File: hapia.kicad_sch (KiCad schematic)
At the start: 89 parts, among them CN1 100nf, CN2 100nf, J1 Conn_ARM_JTAG_SWD_10, J2 USB_C_Receptacle_USB2.0_16P, SW1 SW_Push, SW2 SW_Push, U1 STM32F407VET6, U2 AMS1117-3.3, U3 SRV05-4, Y1 8mhz

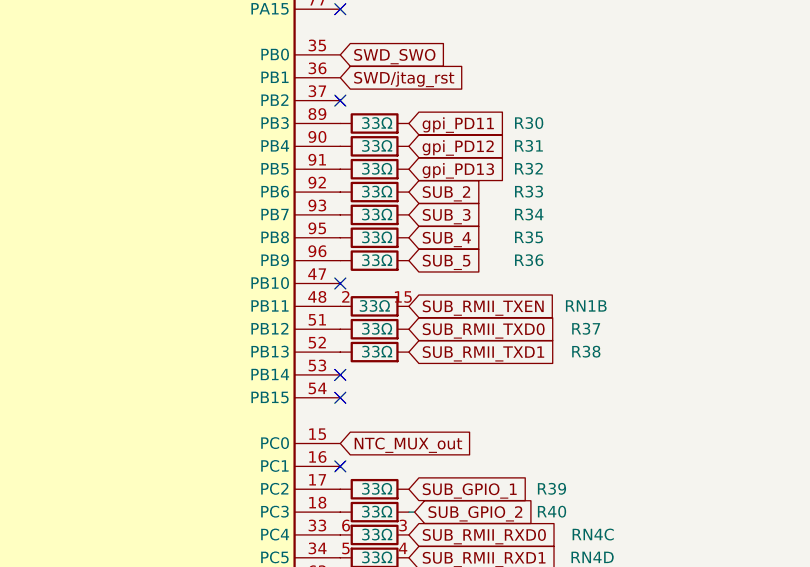
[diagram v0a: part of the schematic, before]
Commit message: 23082026/H
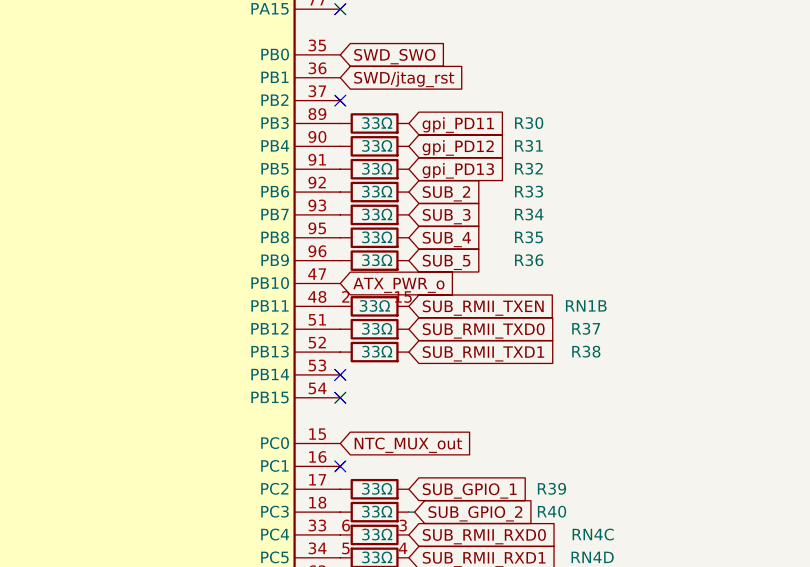
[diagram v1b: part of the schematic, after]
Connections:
- net ATX_PWR_o: now reaches U1.47 (PB10)
- no-connect marks 23 -> 22
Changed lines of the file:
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@@
-	)
-	(no_connect
-		(at 128.27 163.83)
 	)
 	(no_connect
@@
 			(hide yes)
 			(show_name no)
+			(do_not_autoplace no)
+			(effects
+				(font
+					(size 1.27 1.27)
+				)
+				(justify left)
+			)
+		)
+	)
+	(global_label "ATX_PWR_o"
+		(shape input)
+		(at 128.27 163.83 0)
+		(fields_autoplaced yes)
+		(effects
+			(font
+				(size 1.27 1.27)
+			)
+			(justify left)
+		)
+		(property "Intersheetrefs" "${INTERSHEET_REFS}"
+			(at 141.5965 163.83 0)
+			(hide yes)
+			(show_name no)

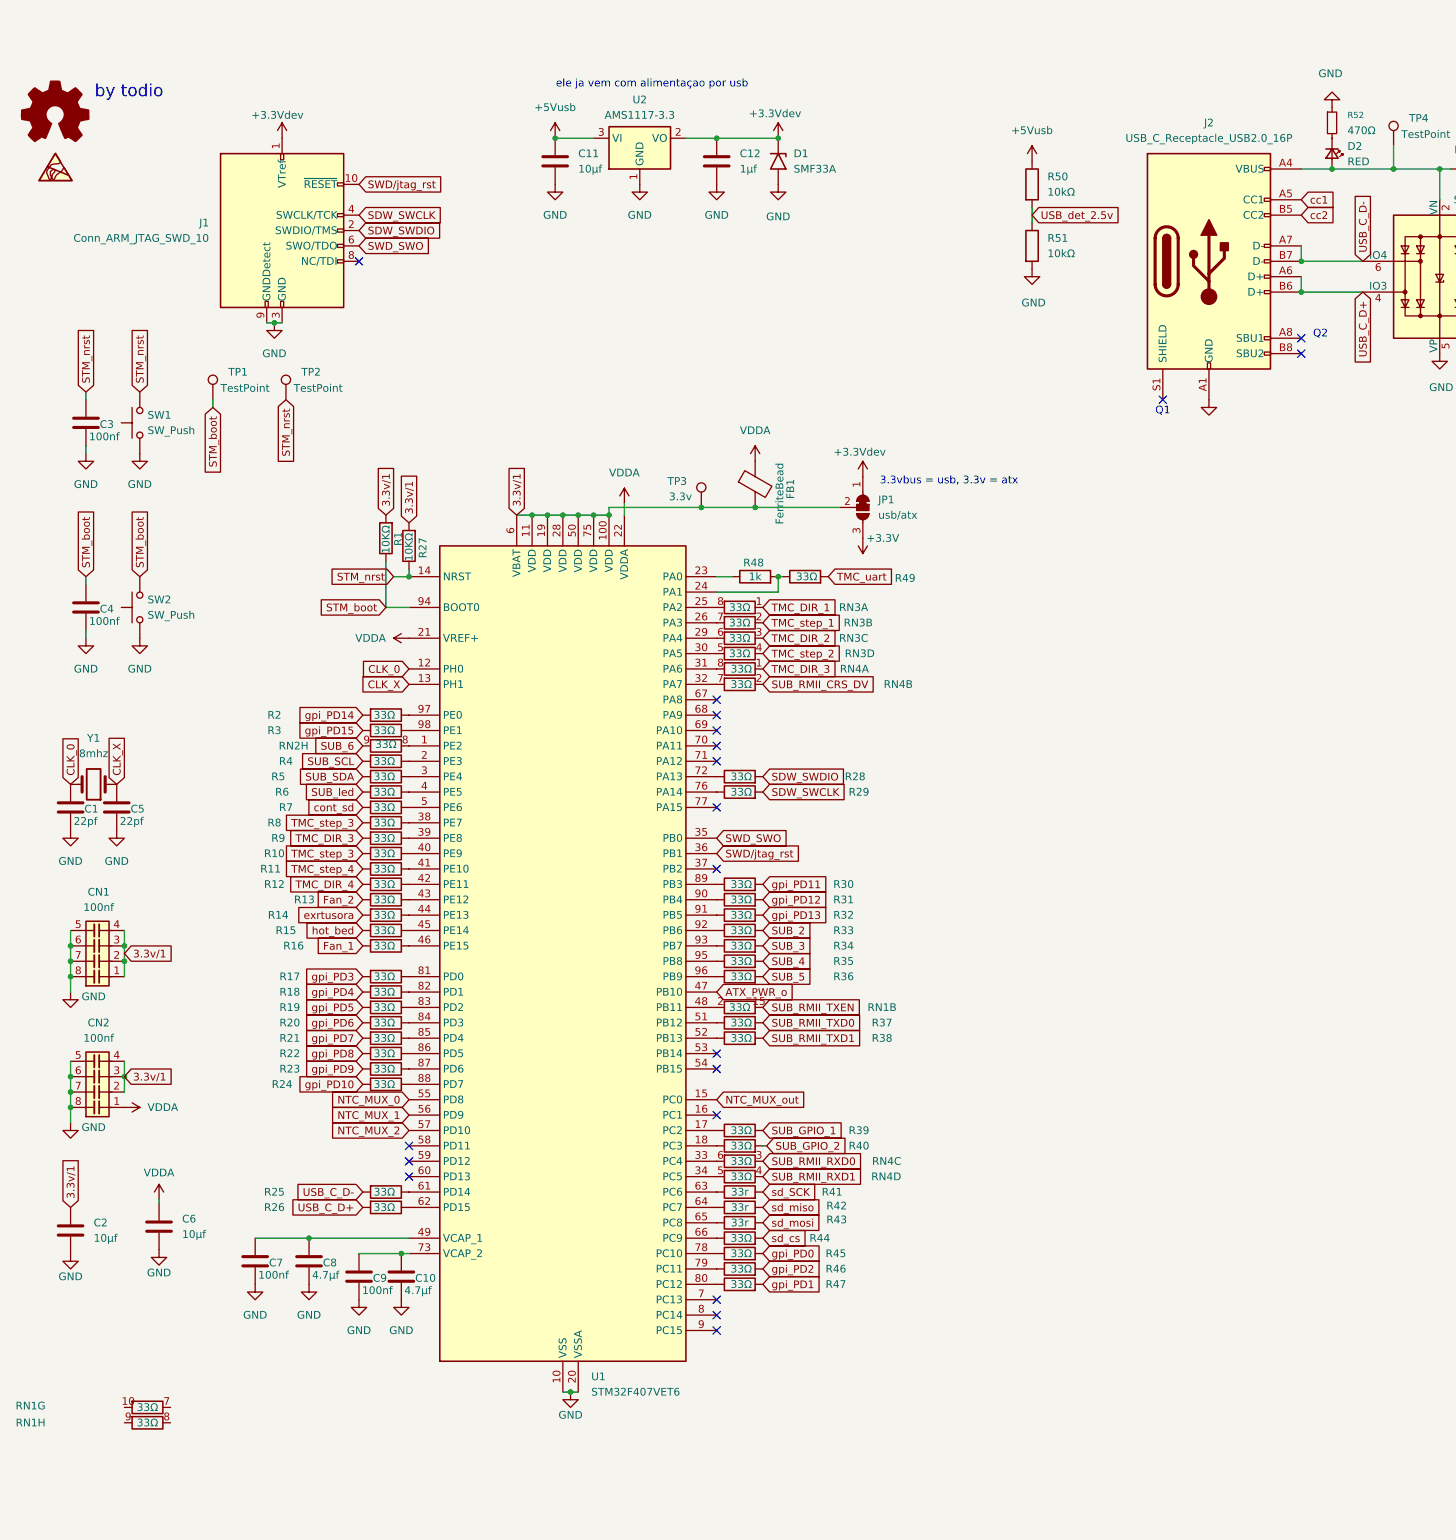
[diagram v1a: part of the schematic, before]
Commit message: 29082026/I
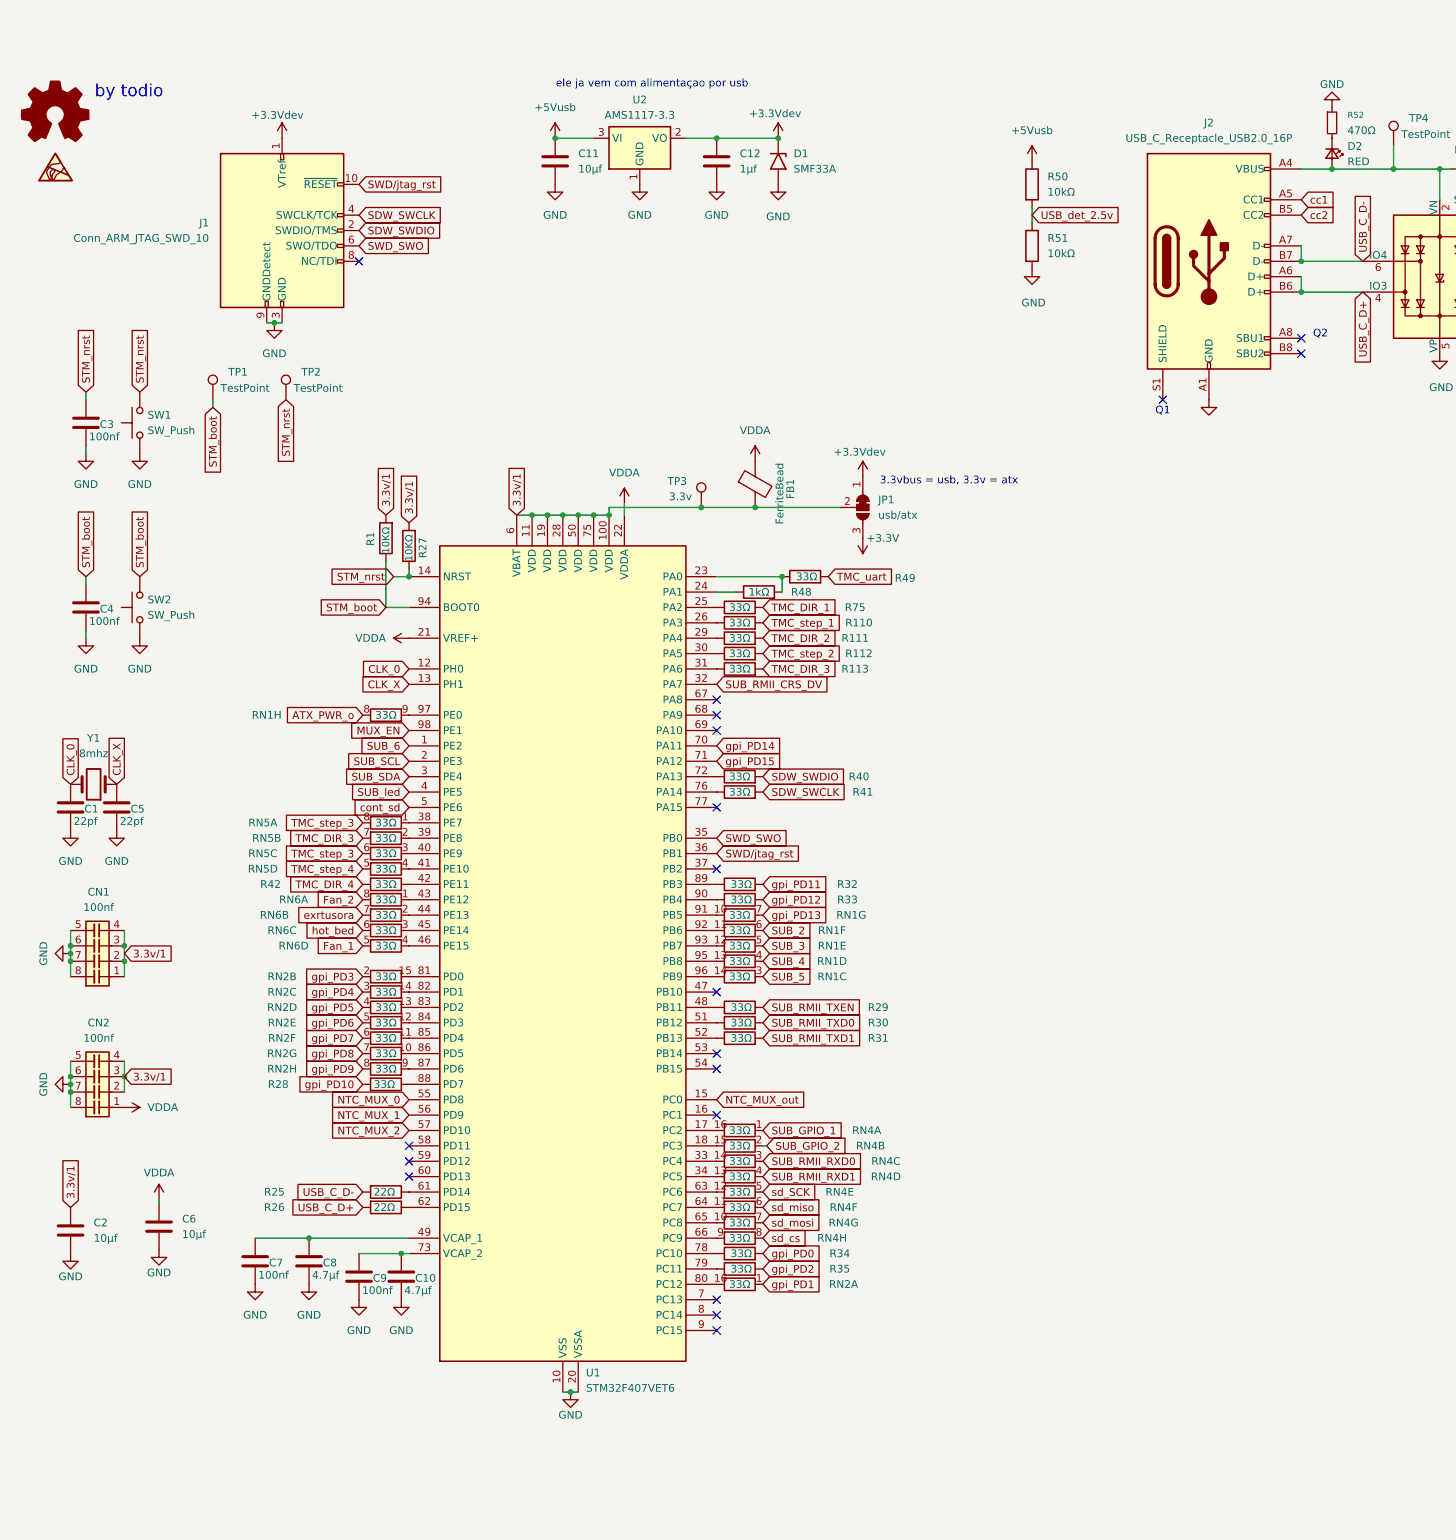
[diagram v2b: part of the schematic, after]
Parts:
- removed R10, R11, R12, R13, R14, R15, R16, R17, R18, R19, R2, R20, R21, R22, R23, R24, R3, R36, R37, R38, R39, R4, R44, R45, R46, R47, R5, R6, R7, R8, R9: 33Ω, symbol Device:R
- removed R43: 33r, symbol Device:R
- removed unit 2 of RN1
- removed RN3, RN4: 33Ω, Resistor_SMD:R_Array_Convex_4x0603, symbol Device:R_Pack04_Split
- added R110, R111, R112, R113, R75: 33Ω, symbol Device:R
- added unit 4 of RN1
- added unit 6 of RN1
- added unit 3 of RN1
- added unit 5 of RN1
- added unit 4 of RN2
- added unit 6 of RN2
- added unit 1 of RN2
- added unit 2 of RN2
- added unit 3 of RN2
- added unit 7 of RN2
- added unit 5 of RN2
- added RN4: 33Ω, symbol Device:R_Pack08_Split
- added RN5, RN6: 33Ω, Resistor_SMD:R_Array_Concave_4x0402, symbol Device:R_Pack04_Split
- C10: footprint (none) -> Capacitor_SMD:C_0603_1608Metric; jlc_pcb: (none) -> C162274; mouser: (none) -> 81-GRM188R61E475KE1D; mpn (none) -> GRM188R61E475KE11D
- C11, C2: footprint (none) -> Capacitor_SMD:C_1206_3216Metric_Pad1.33x1.80mm_HandSolder; jlc_pcb: (none) -> C13585; mouser: (none) -> 187-CL31B106KLK6PNE; mpn (none) -> CL31A106KBHNNNE
- C3, C4, C7, C9: jlc_pcb: C346191 -> C307348; mouser: (none) -> 187-CL10B104KB8WPNC; mpn CL10B104KB8NFNC -> CL10B104KB8WPNC
- C6: footprint (none) -> Capacitor_SMD:C_1206_3216Metric_Pad1.33x1.80mm_HandSolder; Descrição (none) -> esse capacitor e conectado entre o gnd e o vcc(VDDA) do ci 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; jlc_pcb: (none) -> C13585; mouser: (none) -> 187-CL31B106KLK6PNE; mpn (none) -> CL31A106KBHNNNE
- C8: footprint (none) -> Capacitor_SMD:C_0603_1608Metric; Descrição (none) -> capacitor ceramico 4.7uf(µf); jlc_pcb: (none) -> C162274; mouser: (none) -> 81-GRM188R61E475KE1D; mpn (none) -> GRM188R61E475KE11D
- CN1, CN2: jlc_pcb: C346191 -> C307348; mouser: (none) -> 187-CL10B104KB8WPNC; mpn CA0612MRX7R7BB104 -> CL10B104KB8WPNC
- J2: footprint (none) -> Connector_USB:USB_C_Receptacle_HCTL_HC-TYPE-C-16P-01A; jlc_pcb: (none) -> C5150972; mouser: (none) -> 523-12402012E212A; mpn (none) -> 12402012E212A
- R25, R26: value 33Ω -> 22Ω
- R41, R42: value 33r -> 33Ω
- R48: value 1k -> 1kΩ
- RN1, RN2: footprint Resistor_SMD:R_Array_Convex_8x0602 -> (none)
- U1: mouser: (none) -> 511-STM32F407VET6
- U2: mouser: (none) -> 926-LM1117MPX3.3NOPB
- Y1: mouser: (none) -> 815-ABM3-8-D2Y-T
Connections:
- net ATX_PWR_o: now also RN1.8 (R8.1); no longer U1.47 (PB10)
- net Fan_1: now also RN6.5 (R4.2)
- net Fan_2: now also RN6.8 (R1.2)
- net SDW_SWCLK: now also R41.2; no longer R29.2
- net SDW_SWDIO: now also R40.2; no longer R28.2
- net SUB_2: now also RN1.6 (R6.1); no longer R33.2
- net SUB_3: now also RN1.5 (R5.1); no longer R34.2
- net SUB_4: now also RN1.4 (R4.1); no longer R35.2
- net SUB_5: now also RN1.3 (R3.1)
- net SUB_6: now also U1.1 (PE2); no longer RN2.9 (R8.2)
- net SUB_GPIO_1: now also RN4.1 (R1.1)
- net SUB_GPIO_2: now also RN4.2 (R2.1); no longer R40.2
- net SUB_RMII_CRS_DV: now also U1.32 (PA7)
- net SUB_RMII_RXD0: now also RN4.3 (R3.1)
- net SUB_RMII_RXD1: now also RN4.4 (R4.1)
- net SUB_RMII_TXD0: now also R30.2
- net SUB_RMII_TXD1: now also R31.2
- net SUB_RMII_TXEN: now also R29.2
- net SUB_SCL: now also U1.2 (PE3)
- net SUB_SDA: now also U1.3 (PE4)
- net SUB_led: now also U1.4 (PE5)
- net TMC_DIR_1: now also R75.2
- net TMC_DIR_2: now also R111.2
- net TMC_DIR_3: now also R113.2, RN5.7 (R2.2)
- net TMC_DIR_4: now also R42.2
- net TMC_step_1: now also R110.2
- net TMC_step_2: now also R112.2
- net TMC_step_3: now also RN5.6 (R3.2), RN5.8 (R1.2)
- net TMC_step_4: now also RN5.5 (R4.2)
- net cont_sd: now also U1.5 (PE6)
- net exrtusora: now also RN6.7 (R2.2)
- net gpi_PD0: now also R34.2
- net gpi_PD1: now also RN2.1 (R1.1)
- net gpi_PD10: now also R28.2
- net gpi_PD11: now also R32.2; no longer R30.2
- net gpi_PD12: now also R33.2; no longer R31.2
- net gpi_PD13: now also RN1.7 (R7.1); no longer R32.2
- net gpi_PD14: now also U1.70 (PA11)
- net gpi_PD15: now also U1.71 (PA12)
- net gpi_PD2: now also R35.2
- net gpi_PD3: now also RN2.2 (R2.1)
- net gpi_PD4: now also RN2.3 (R3.1)
- net gpi_PD5: now also RN2.4 (R4.1)
- net gpi_PD6: now also RN2.5 (R5.1)
- net gpi_PD7: now also RN2.6 (R6.1)
- net gpi_PD8: now also RN2.7 (R7.1)
- net gpi_PD9: now also RN2.8 (R8.1)
- net hot_bed: now also RN6.6 (R3.2)
- net sd_SCK: now also RN4.5 (R5.1); no longer R41.2
- net sd_cs: now also RN4.8 (R8.1)
- net sd_miso: now also RN4.6 (R6.1); no longer R42.2
- net sd_mosi: now also RN4.7 (R7.1)
- net at U1.52 (PB13): now also R31.1
- net at U1.43 (PE12): now also RN6.1 (R1.1)
- net at U1.65 (PC8): now also RN4.10 (R7.2)
- net at U1.79 (PC11): now also R35.1
- net at U1.38 (PE7): now also RN5.1 (R1.1)
- net at U1.48 (PB11): now also R29.1
- net at U1.85 (PD4): now also RN2.11 (R6.2)
- net at U1.18 (PC3): now also RN4.15 (R2.2); no longer R40.1
- net at U1.26 (PA3): now also R110.1
- net at U1.51 (PB12): now also R30.1
- net at U1.89 (PB3): now also R32.1; no longer R30.1
- net at U1.88 (PD7): now also R28.1
- net at R48.1: now also U1.24 (PA1); no longer U1.23 (PA0)
- net at R48.2, R49.1: now also U1.23 (PA0); no longer U1.24 (PA1)
- net at U1.17 (PC2): now also RN4.16 (R1.2)
- net at U1.25 (PA2): now also R75.1
- net at U1.29 (PA4): now also R111.1
- net at U1.30 (PA5): now also R112.1
- net at U1.31 (PA6): now also R113.1
- net at U1.33 (PC4): now also RN4.14 (R3.2)
- net at U1.34 (PC5): now also RN4.13 (R4.2)
- net at U1.39 (PE8): now also RN5.2 (R2.1)
- net at U1.40 (PE9): now also RN5.3 (R3.1)
- net at U1.41 (PE10): now also RN5.4 (R4.1)
- net at U1.42 (PE11): now also R42.1
- net at U1.44 (PE13): now also RN6.2 (R2.1)
- net at U1.45 (PE14): now also RN6.3 (R3.1)
- net at U1.46 (PE15): now also RN6.4 (R4.1)
- net at R41.1: now also U1.76 (PA14); no longer U1.63 (PC6)
- net at U1.64 (PC7): now also RN4.11 (R6.2); no longer R42.1
- net at U1.66 (PC9): now also RN4.9 (R8.2)
- net at U1.72 (PA13): now also R40.1; no longer R28.1
- net at U1.78 (PC10): now also R34.1
- net at U1.80 (PC12): now also RN2.16 (R1.2)
- net at U1.81 (PD0): now also RN2.15 (R2.2)
- net at U1.82 (PD1): now also RN2.14 (R3.2)
- net at U1.83 (PD2): now also RN2.13 (R4.2)
- net at U1.84 (PD3): now also RN2.12 (R5.2)
- net at U1.86 (PD5): now also RN2.10 (R7.2)
- net at U1.87 (PD6): now also RN2.9 (R8.2)
- net at U1.90 (PB4): now also R33.1; no longer R31.1
- net at U1.91 (PB5): now also RN1.10 (R7.2); no longer R32.1
- net at U1.92 (PB6): now also RN1.11 (R6.2); no longer R33.1
- net at U1.93 (PB7): now also RN1.12 (R5.2); no longer R34.1
- net at U1.95 (PB8): now also RN1.13 (R4.2); no longer R35.1
- net at U1.96 (PB9): now also RN1.14 (R3.2)
- net at U1.97 (PE0): now also RN1.9 (R8.2)
- net MUX_EN: now reaches U1.98 (PE1)
- new net: RN4.12 (R5.2), U1.63 (PC6)
- no-connect marks 22 -> 21
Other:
- moved on the sheet: R48
